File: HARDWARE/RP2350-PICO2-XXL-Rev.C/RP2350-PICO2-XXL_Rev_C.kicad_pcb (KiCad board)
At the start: 4 copper layers, 29 x 51 mm, 85 parts, among them Q1 Q12MHz/18pF/30ppm/4P/3.2x2.5m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, U1 W25Q128JVSIQ(SOIC-8_208mils), U2 TPS62A02ADRLR(SOT-563-6), U3 RP2350B(QFN-80_10.00x10.00x0.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, U4 NA(W25Q128JVSIQ(SOIC-8_208mil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, U5 APS6404L-3SQR-SN(SOIC-8_150mi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

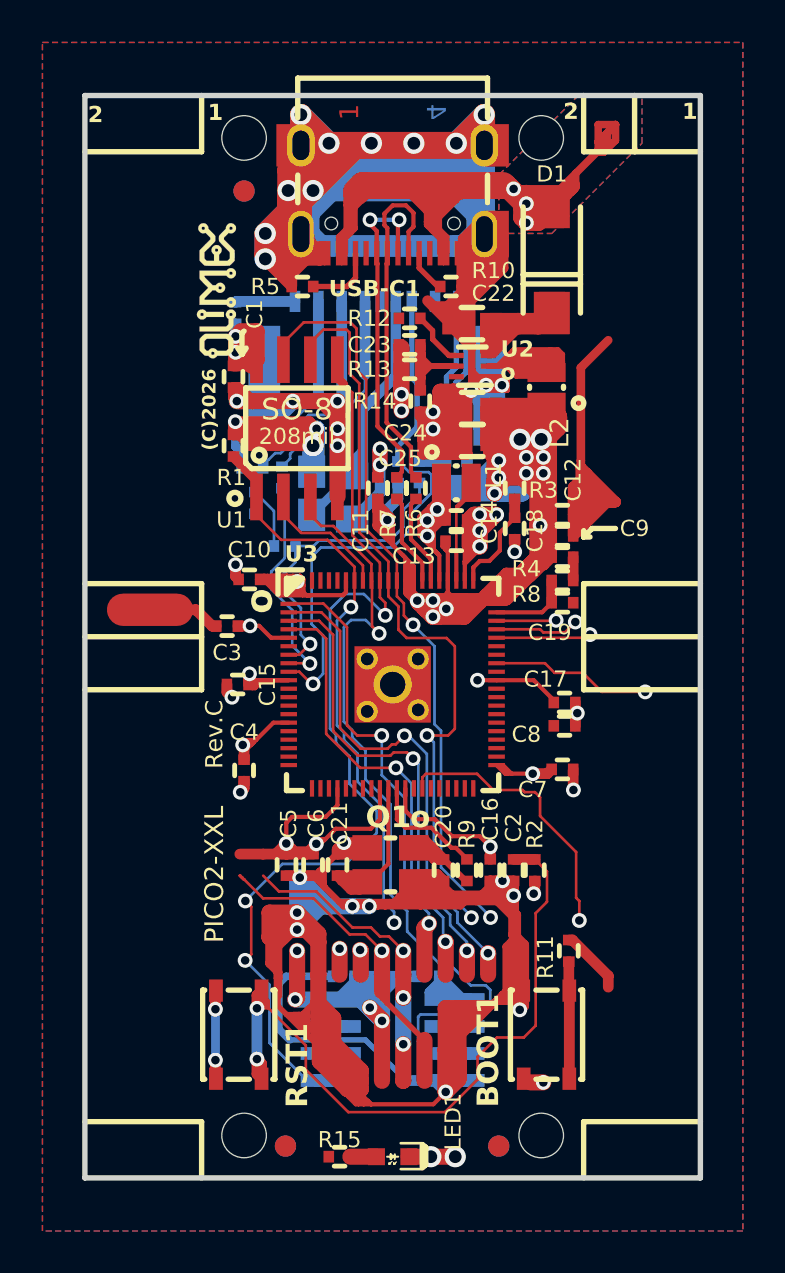
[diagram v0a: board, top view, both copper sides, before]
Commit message: cleaning up
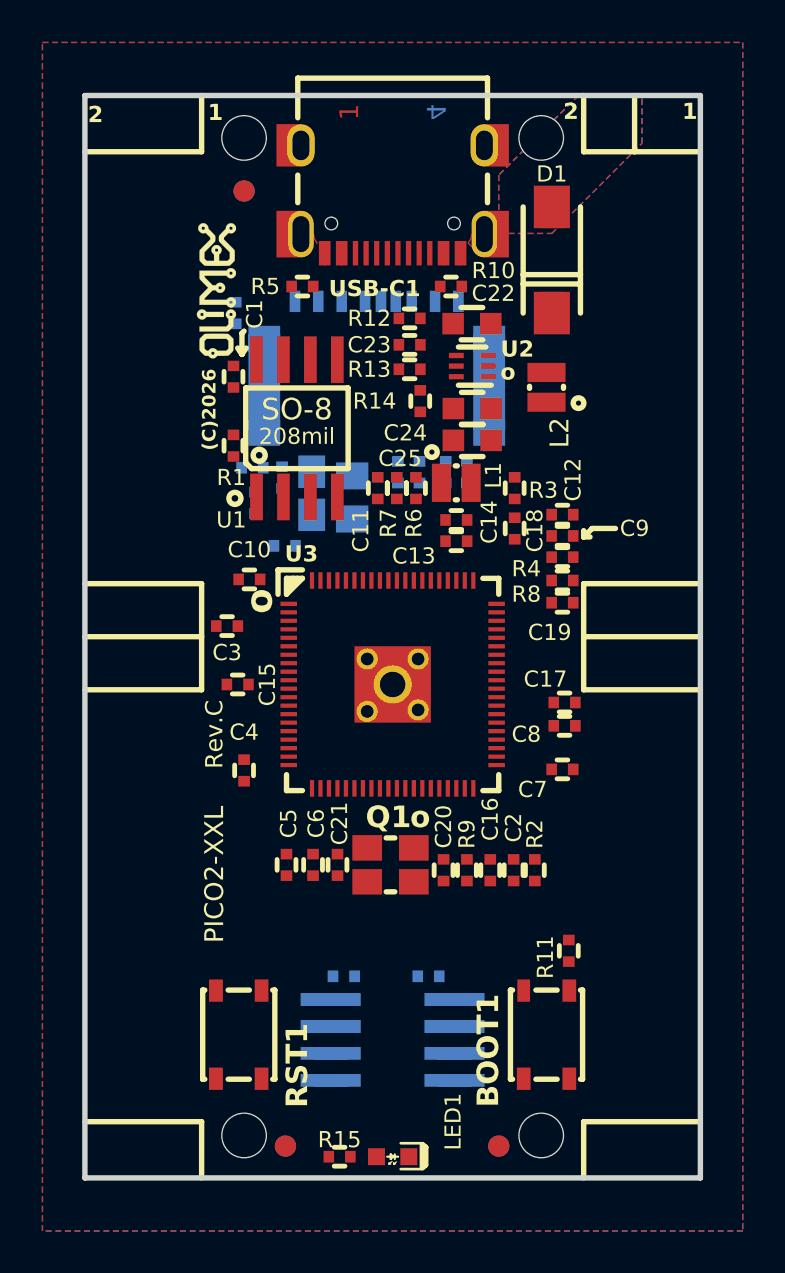
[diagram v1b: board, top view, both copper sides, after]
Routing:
- net GND: track 593.4 -> 0.00 mm, vias 47 -> 0
- net +3.3V: track 385.8 -> 0.00 mm, vias 33 -> 0
- net /+1V1: track 112.2 -> 0.00 mm, vias 6 -> 0
- net VBUS: track 97.4 -> 0.00 mm, vias 3 -> 0
- net /GPIO3\I2C1_SCL: track 61.6 -> 0.00 mm, vias 1 -> 0
- net /GPIO2\I2C1_SDA: track 56.3 -> 0.00 mm, vias 3 -> 0
- net /GPIO47: track 47.5 -> 0.00 mm, vias 1 -> 0
- net /QSPI_SD0: track 46.0 -> 0.00 mm, vias 3 -> 0
- net /QSPI_CLK: track 44.1 -> 0.00 mm, vias 2 -> 0
- net /GPIO0\UART0_TX: track 44.0 -> 0.00 mm, vias 1 -> 0
- net /GPIO1\UART0_RX: track 43.7 -> 0.00 mm, vias 1 -> 0
- net /QSPI_CSn: track 42.0 -> 0.00 mm, vias 2 -> 0
- net /QSPI_SD3: track 41.7 -> 0.00 mm, vias 2 -> 0
- net /QSPI_SD2: track 38.7 -> 0.00 mm, vias 1 -> 0
- net /RUN: track 36.7 -> 0.00 mm, vias 2 -> 0
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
